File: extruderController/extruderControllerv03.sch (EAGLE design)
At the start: 74 parts, among them IC1 LM1117MPX-5.0, IC2 MAX3467CPA, IC3 ATMEGA2561-16AU, IC4 ULN2003AD, J8 615016137621, Q2 PH7030L, Q3 PH7030L, Q4 PH7030L, Q5 PH7030L, Q6 PH7030L, X1 22-23-2081, X2 22-23-2081, X3 22-23-2101, X6 22-23-2041, X8 22-23-2031, X9 22-23-2031

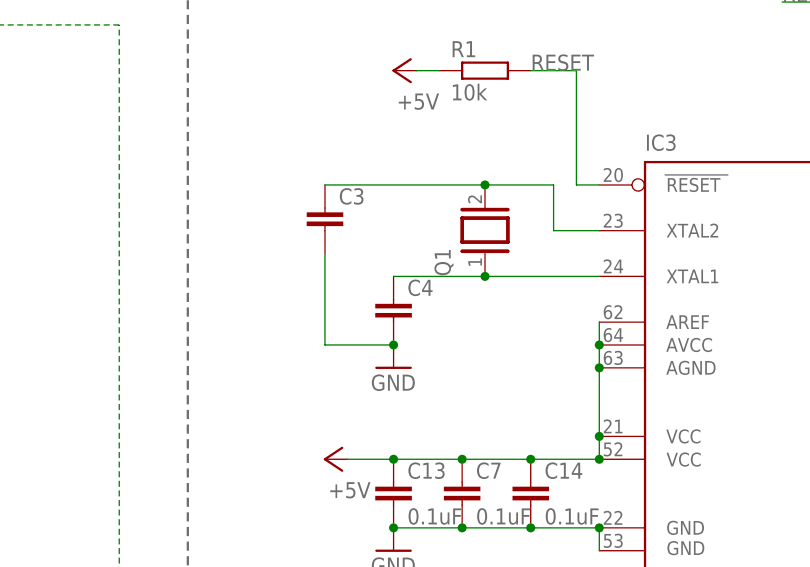
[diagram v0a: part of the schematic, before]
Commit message: j
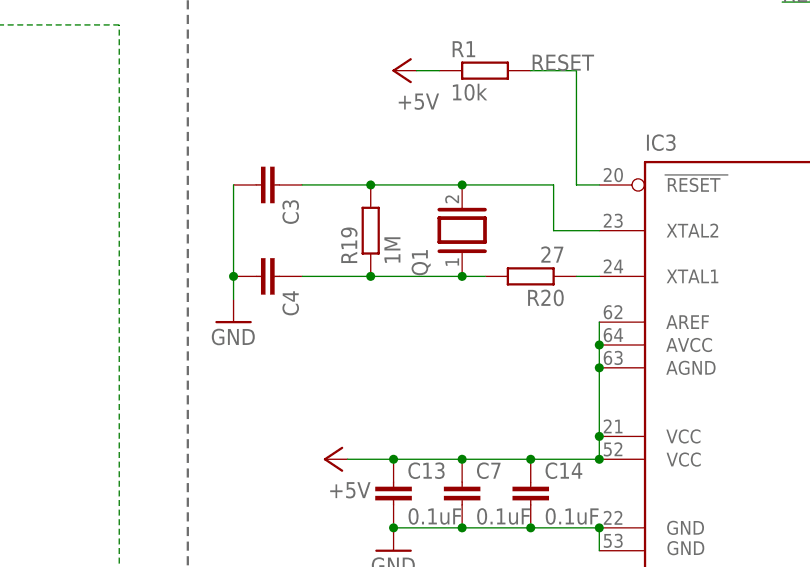
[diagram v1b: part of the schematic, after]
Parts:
- added R19: 1M, rcl:R-EU_R0805
- added R20: 27, rcl:R-EU_R0805
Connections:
- new net N$35: IC3.XTAL1, R20.1
- net N$19: now also R19.2
- net N$20: now also R19.1, R20.2; no longer IC3.XTAL1
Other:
- moved on the sheet: C3, C4, Q1
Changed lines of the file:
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@@
 <?xml version="1.0" encoding="utf-8"?>
 <!DOCTYPE eagle SYSTEM "eagle.dtd">
-<eagle version="9.3.1">
+<eagle version="9.2.2">
 <drawing>
 <settings>
@@
 <part name="GND24" library="supply1" library_urn="urn:adsk.eagle:library:371" deviceset="GND" device=""/>
 <part name="P+34" library="supply1" library_urn="urn:adsk.eagle:library:371" deviceset="+5V" device=""/>
+<part name="R19" library="rcl" library_urn="urn:adsk.eagle:library:334" deviceset="R-EU_" device="R0805" package3d_urn="urn:adsk.eagle:package:23553/2" value="1M"/>
+<part name="R20" library="rcl" library_urn="urn:adsk.eagle:library:334" deviceset="R-EU_" device="R0805" package3d_urn="urn:adsk.eagle:package:23553/2" value="27"/>
 </parts>
 <sheets>
@@
 <attribute name="VALUE" x="-195.58" y="93.98" size="1.778" layer="96" rot="R180"/>
 </instance>
-<instance part="Q1" gate="G$1" x="-76.2" y="121.92" smashed="yes" rot="R90">
-<attribute name="NAME" x="-80.01" y="116.84" size="1.778" layer="95" rot="R90"/>
-<attribute name="VALUE" x="-71.12" y="116.84" size="1.778" layer="96" rot="R90"/>
+<instance part="Q1" gate="G$1" x="-78.74" y="121.92" smashed="yes" rot="R90">
+<attribute name="NAME" x="-82.55" y="116.84" size="1.778" layer="95" rot="R90"/>
+<attribute name="VALUE" x="-73.66" y="116.84" size="1.778" layer="96" rot="R90"/>
 </instance>
 <instance part="P+8" gate="1" x="-93.98" y="96.52" smashed="yes" rot="R90">
@@
 <attribute name="NAME" x="-142.24" y="165.862" size="1.524" layer="95" rot="R180"/>
 </instance>
-<instance part="C3" gate="G$1" x="-93.98" y="124.46" smashed="yes">
-<attribute name="NAME" x="-92.456" y="124.841" size="1.778" layer="95"/>
-<attribute name="VALUE" x="-92.456" y="119.761" size="1.778" layer="96"/>
-</instance>
-<instance part="C4" gate="G$1" x="-86.36" y="114.3" smashed="yes">
-<attribute name="NAME" x="-84.836" y="114.681" size="1.778" layer="95"/>
-<attribute name="VALUE" x="-84.836" y="109.601" size="1.778" layer="96"/>
-</instance>
-<instance part="GND13" gate="1" x="-86.36" y="106.68" smashed="yes">
-<attribute name="VALUE" x="-88.9" y="104.14" size="1.778" layer="96"/>
+<instance part="C3" gate="G$1" x="-99.06" y="127" smashed="yes" rot="R270">
+<attribute name="NAME" x="-98.679" y="125.476" size="1.778" layer="95" rot="R270"/>
+<attribute name="VALUE" x="-103.759" y="125.476" size="1.778" layer="96" rot="R270"/>
+</instance>
+<instance part="C4" gate="G$1" x="-99.06" y="116.84" smashed="yes" rot="R270">
+<attribute name="NAME" x="-98.679" y="115.316" size="1.778" layer="95" rot="R270"/>
+<attribute name="VALUE" x="-103.759" y="115.316" size="1.778" layer="96" rot="R270"/>
+</instance>
+<instance part="GND13" gate="1" x="-104.14" y="111.76" smashed="yes">
+<attribute name="VALUE" x="-106.68" y="109.22" size="1.778" layer="96"/>
 </instance>
 <instance part="R1" gate="G$1" x="-76.2" y="139.7" smashed="yes">
@@
 <instance part="P+34" gate="1" x="83.82" y="236.22" smashed="yes" rot="R270">
 <attribute name="VALUE" x="78.74" y="238.76" size="1.778" layer="96"/>
+</instance>
+<instance part="R19" gate="G$1" x="-88.9" y="121.92" smashed="yes" rot="R90">
+<attribute name="NAME" x="-90.3986" y="118.11" size="1.778" layer="95" rot="R90"/>
+<attribute name="VALUE" x="-85.598" y="118.11" size="1.778" layer="96" rot="R90"/>
+</instance>
+<instance part="R20" gate="G$1" x="-71.12" y="116.84" smashed="yes" rot="R180">
+<attribute name="NAME" x="-67.31" y="115.3414" size="1.778" layer="95" rot="R180"/>
+<attribute name="VALUE" x="-67.31" y="120.142" size="1.778" layer="96" rot="R180"/>
 </instance>
 </instances>
@@
 <pinref part="GND12" gate="1" pin="GND"/>
 <wire x1="-12.7" y1="147.32" x2="-15.24" y2="147.32" width="0.1524" layer="91"/>
-</segment>
-<segment>
-<pinref part="C4" gate="G$1" pin="2"/>
-<pinref part="GND13" gate="1" pin="GND"/>
-<pinref part="C3" gate="G$1" pin="2"/>
-<wire x1="-93.98" y1="119.38" x2="-93.98" y2="109.22" width="0.1524" layer="91"/>
-<wire x1="-93.98" y1="109.22" x2="-86.36" y2="109.22" width="0.1524" layer="91"/>
-<junction x="-86.36" y="109.22"/>
 </segment>
 <segment>
@@
 <pinref part="J1" gate="G$1" pin="1"/>
 <pinref part="GND24" gate="1" pin="GND"/>
+</segment>
+<segment>
+<pinref part="GND13" gate="1" pin="GND"/>
+<pinref part="C4" gate="G$1" pin="2"/>
+<wire x1="-104.14" y1="114.3" x2="-104.14" y2="116.84" width="0.1524" layer="91"/>
+<pinref part="C3" gate="G$1" pin="2"/>
+<wire x1="-104.14" y1="127" x2="-104.14" y2="116.84" width="0.1524" layer="91"/>
+<junction x="-104.14" y="116.84"/>
 </segment>
 </net>
@@
 <wire x1="-68.58" y1="121.92" x2="-68.58" y2="127" width="0.1524" layer="91"/>
 <pinref part="Q1" gate="G$1" pin="2"/>
-<wire x1="-68.58" y1="127" x2="-76.2" y2="127" width="0.1524" layer="91"/>
+<wire x1="-68.58" y1="127" x2="-78.74" y2="127" width="0.1524" layer="91"/>
 <pinref part="C3" gate="G$1" pin="1"/>
-<wire x1="-93.98" y1="127" x2="-76.2" y2="127" width="0.1524" layer="91"/>
-<junction x="-76.2" y="127"/>
+<wire x1="-96.52" y1="127" x2="-88.9" y2="127" width="0.1524" layer="91"/>
+<junction x="-78.74" y="127"/>
+<pinref part="R19" gate="G$1" pin="2"/>
+<wire x1="-88.9" y1="127" x2="-78.74" y2="127" width="0.1524" layer="91"/>
+<junction x="-88.9" y="127"/>
 </segment>
 </net>
@@
 <pinref part="C4" gate="G$1" pin="1"/>
 <pinref part="Q1" gate="G$1" pin="1"/>
-<wire x1="-86.36" y1="116.84" x2="-76.2" y2="116.84" width="0.1524" layer="91"/>
-<pinref part="IC3" gate="G$1" pin="XTAL1"/>
-<wire x1="-63.5" y1="116.84" x2="-76.2" y2="116.84" width="0.1524" layer="91"/>
-<junction x="-76.2" y="116.84"/>
+<wire x1="-96.52" y1="116.84" x2="-88.9" y2="116.84" width="0.1524" layer="91"/>
+<pinref part="R20" gate="G$1" pin="2"/>
+<wire x1="-88.9" y1="116.84" x2="-78.74" y2="116.84" width="0.1524" layer="91"/>
+<wire x1="-76.2" y1="116.84" x2="-78.74" y2="116.84" width="0.1524" layer="91"/>
+<junction x="-78.74" y="116.84"/>
+<pinref part="R19" gate="G$1" pin="1"/>
+<junction x="-88.9" y="116.84"/>
 </segment>
 </net>
@@
 </segment>
 </net>
+<net name="N$35" class="0">
+<segment>
+<pinref part="R20" gate="G$1" pin="1"/>
+<pinref part="IC3" gate="G$1" pin="XTAL1"/>
+<wire x1="-66.04" y1="116.84" x2="-63.5" y2="116.84" width="0.1524" layer="91"/>
+</segment>
+</net>
